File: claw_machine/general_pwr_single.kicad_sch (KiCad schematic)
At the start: 6 parts, among them J33 Conn_01x02_Pin, J37 Screw_Terminal_01x02, Q1 AO3400A

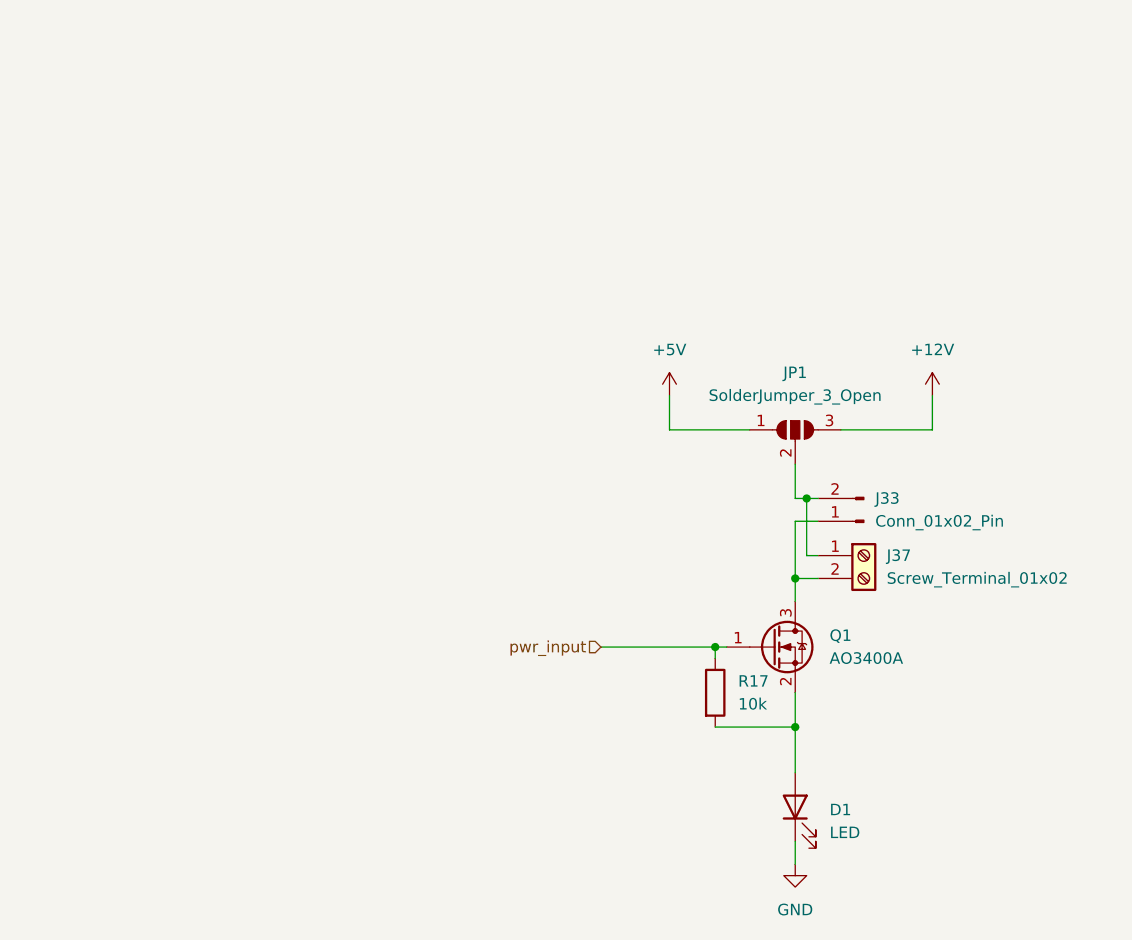
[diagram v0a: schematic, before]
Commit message: Rework schematic
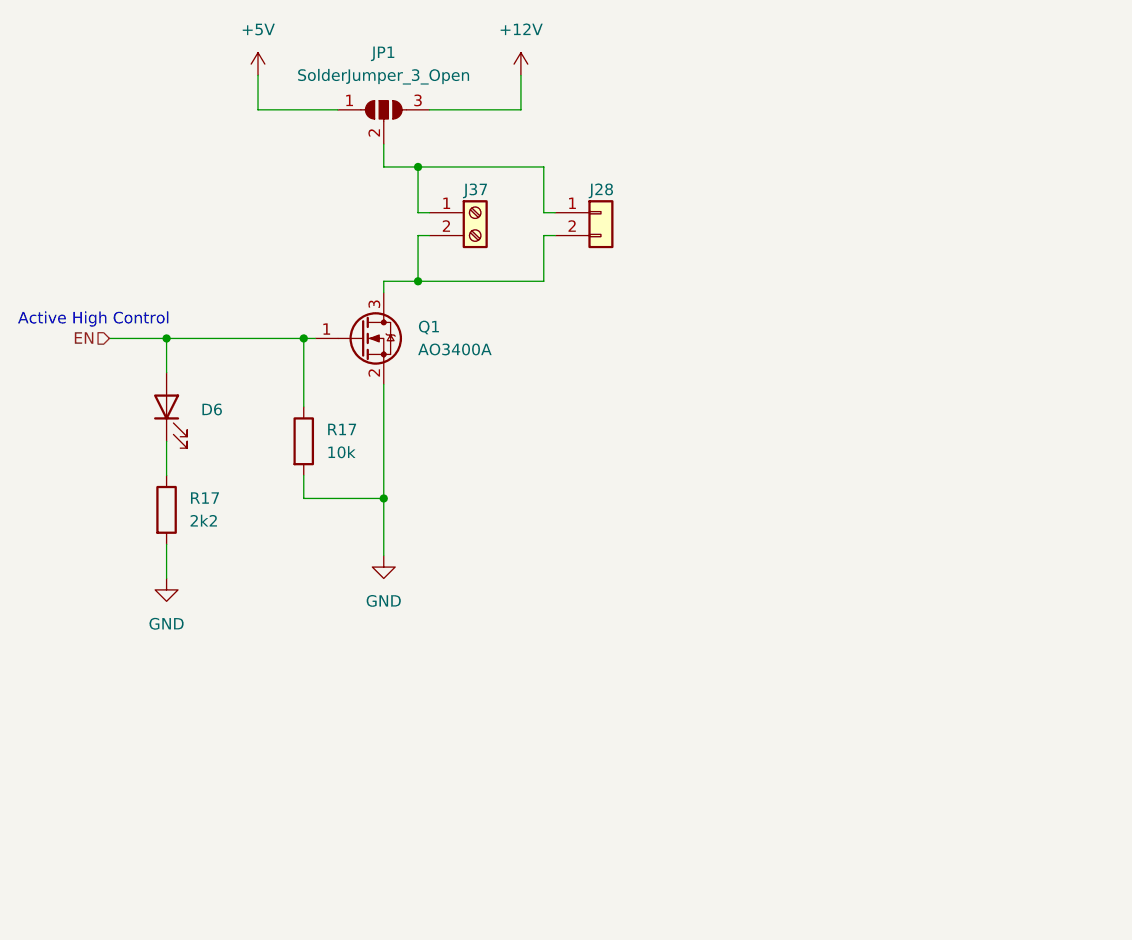
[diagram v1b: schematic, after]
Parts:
- removed D1: LED, LED_THT:LED_D1.8mm_W1.8mm_H2.4mm_Horizontal_O1.27mm_Z1.6mm, symbol Device:LED
- removed J33: Conn_01x02_Pin, symbol Connector:Conn_01x02_Pin
- added D6: LED, LED_THT:LED_D1.8mm_W1.8mm_H2.4mm_Horizontal_O1.27mm_Z1.6mm, symbol Device:LED
- added J28: Conn_01x02, symbol Connector_Generic:Conn_01x02
- added R17: 2k2, Resistor_SMD:R_0805_2012Metric_Pad1.20x1.40mm_HandSolder, symbol Device:R
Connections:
- net GND: now also Q1.2 (S), R17.2, R17.2
- net at J37.2 (Pin_2), Q1.3 (D): now also J28.2 (Pin_2)
- net at J37.1 (Pin_1), JP1.2 (C): now also J28.1 (Pin_1)
- net pwr_input renamed EN
- net EN: now also D6.2 (A)
- new net: D6.1 (K), R17.1
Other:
- note added: "Active High Control"
- moved on the sheet: J37, JP1, Q1, R17
